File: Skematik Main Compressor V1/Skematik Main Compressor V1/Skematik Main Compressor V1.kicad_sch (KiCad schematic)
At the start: 4 parts, among them J1 Conn_01x04_Pin, U1 ESP32-WROOM-32UE

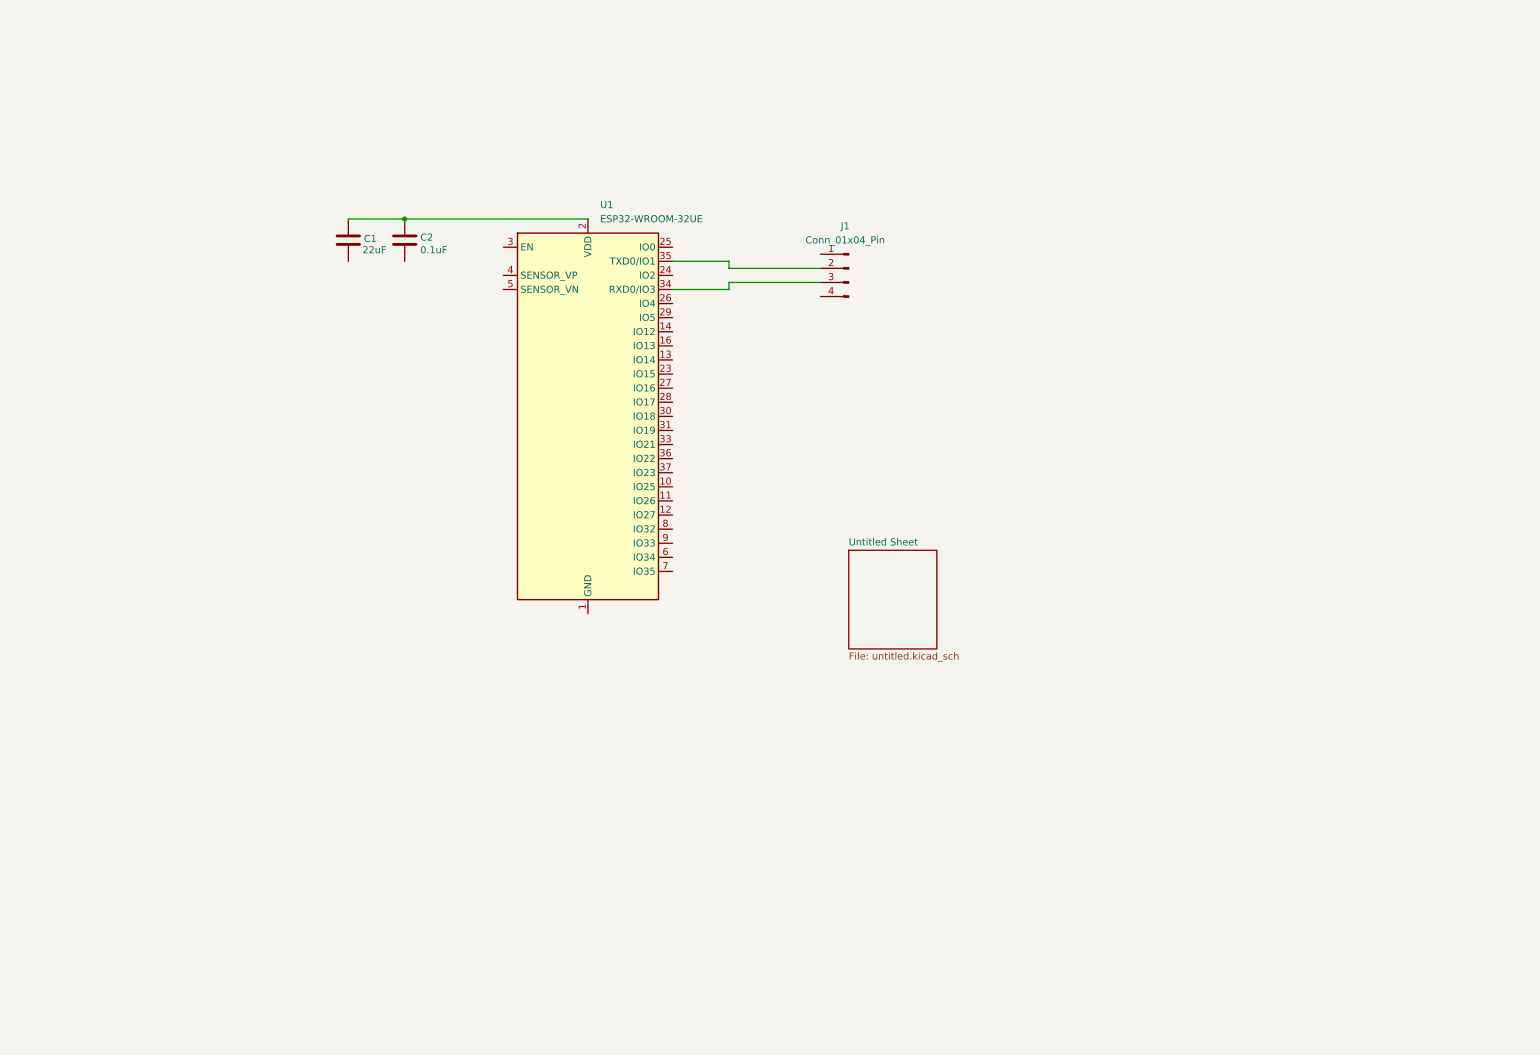
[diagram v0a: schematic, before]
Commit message: Update Main
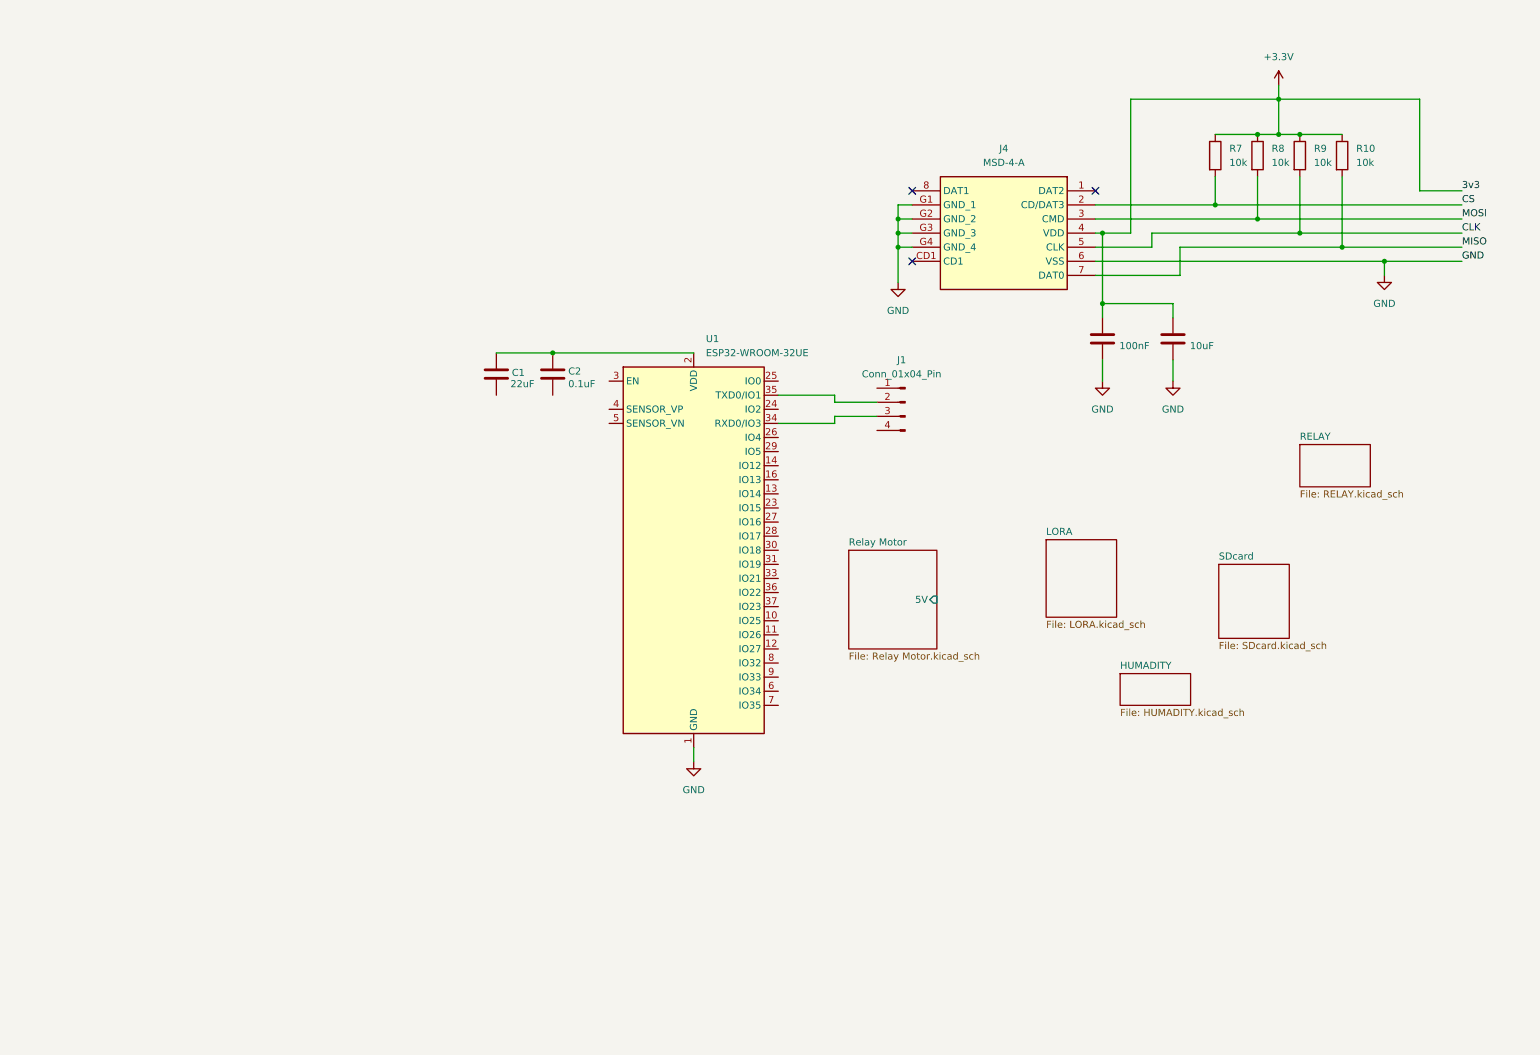
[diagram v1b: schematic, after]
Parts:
- added C5: 100nF, Capacitor_SMD:C_0504_1310Metric_Pad0.83x1.28mm_HandSolder, symbol Device:C
- added C6: 10uF, Capacitor_SMD:C_0504_1310Metric_Pad0.83x1.28mm_HandSolder, symbol Device:C
- added J4: MSD-4-A, MSD4A, symbol MSD-4-A:MSD-4-A
- added R10, R7, R8, R9: 10k, Resistor_SMD:R_0402_1005Metric_Pad0.72x0.64mm_HandSolder, symbol Device:R
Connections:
- net GND: now reaches U1.1 (GND), U1.15 (GND), U1.38 (GND), U1.39 (GND)
- net GND: now also C5.2, C6.2, J4.6 (VSS), J4.G1 (GND_1), J4.G2 (GND_2), J4.G3 (GND_3), J4.G4 (GND_4)
- new net +3.3V: C5.1, C6.1, J4.4 (VDD), R10.1, R7.1, R8.1, R9.1
- new net CLK: J4.5 (CLK), R9.2
- new net CS: J4.2 (CD/DAT3), R7.2
- new net MISO: J4.7 (DAT0), R10.2
- new net MOSI: J4.3 (CMD), R8.2
- no-connect marks 0 -> 3
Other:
- sheet Untitled Sheet renamed Relay Motor
- added sheet HUMADITY (HUMADITY.kicad_sch)
- added sheet LORA (LORA.kicad_sch)
- added sheet RELAY (RELAY.kicad_sch)
- added sheet SDcard (SDcard.kicad_sch)
- sheet Relay Motor: file untitled.kicad_sch -> Relay Motor.kicad_sch
- sheet Relay Motor ports: added 5V; removed none
- moved on the sheet: C1, C2, J1, U1

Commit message: Penambahan Skematik Main Compressor V1
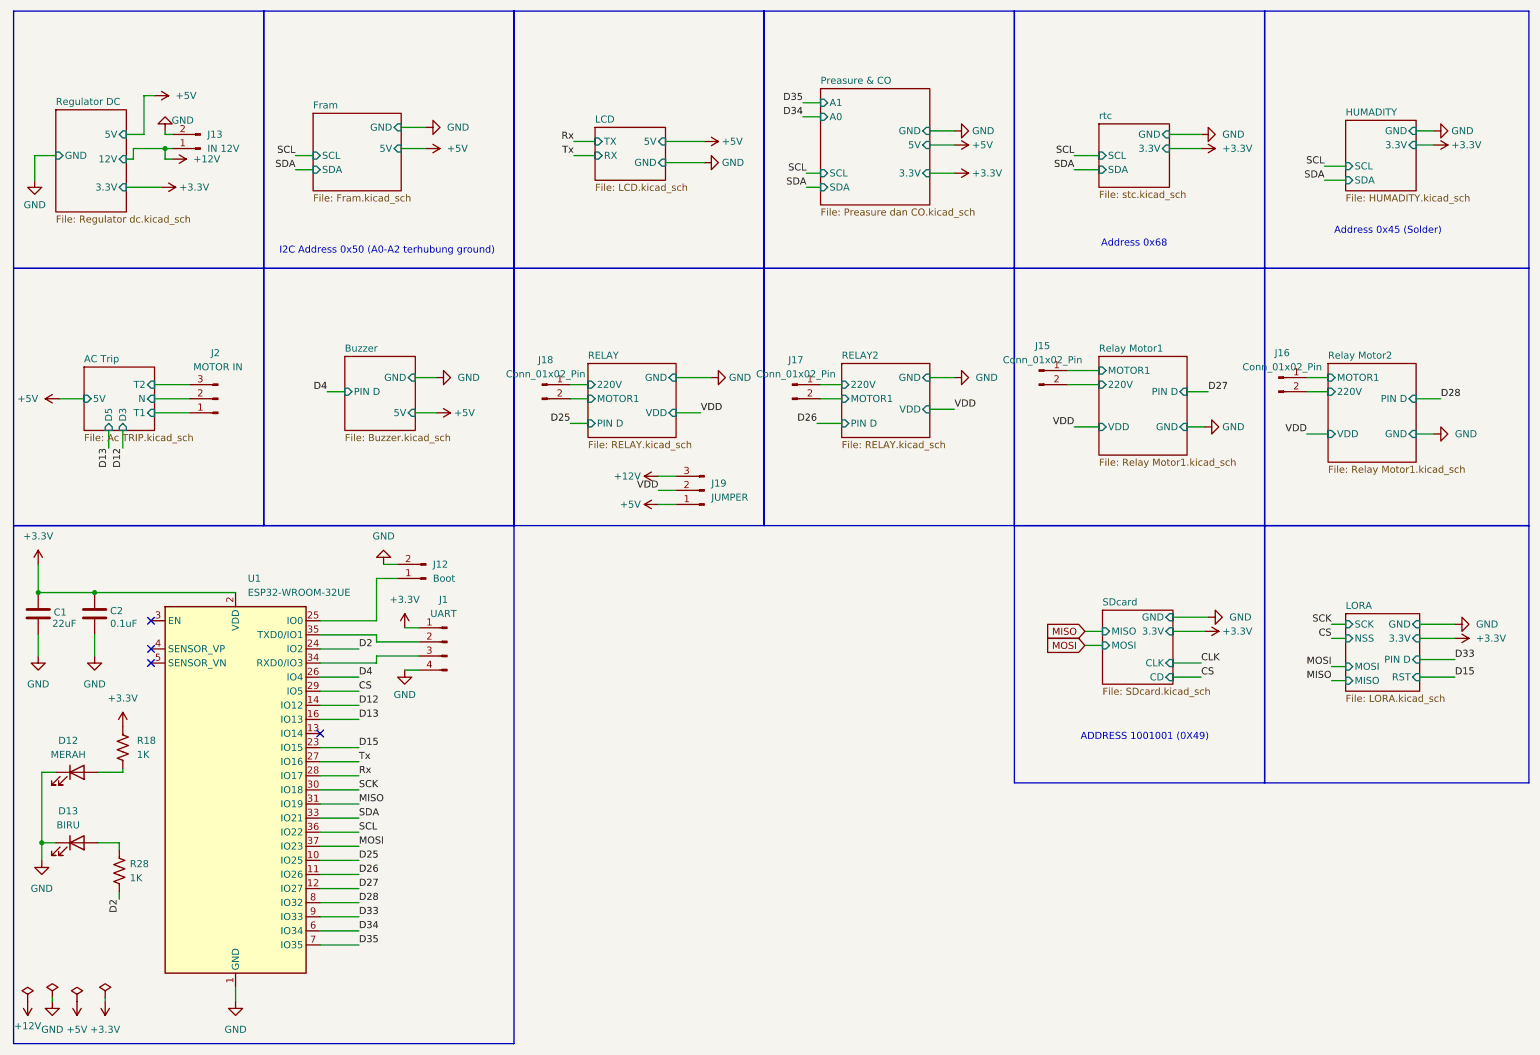
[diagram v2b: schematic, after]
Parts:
- removed C5: 100nF, Capacitor_SMD:C_0504_1310Metric_Pad0.83x1.28mm_HandSolder, symbol Device:C
- removed C6: 10uF, Capacitor_SMD:C_0504_1310Metric_Pad0.83x1.28mm_HandSolder, symbol Device:C
- removed J4: MSD-4-A, MSD4A, symbol MSD-4-A:MSD-4-A
- removed R10, R7, R8, R9: 10k, Resistor_SMD:R_0402_1005Metric_Pad0.72x0.64mm_HandSolder, symbol Device:R
- added D12: MERAH, LED_SMD:LED_0402_1005Metric_Pad0.77x0.64mm_HandSolder, symbol Device:LED
- added D13: BIRU, LED_SMD:LED_0402_1005Metric_Pad0.77x0.64mm_HandSolder, symbol Device:LED
- added J12: Boot, Connector_PinHeader_2.54mm:PinHeader_1x02_P2.54mm_Vertical, symbol Connector:Conn_01x02_Pin
- added J13: IN 12V, Connector_Molex:Molex_KK-396_A-41791-0002_1x02_P3.96mm_Vertical, symbol Connector:Conn_01x02_Pin
- added J15, J16, J17, J18: Conn_01x02_Pin, Connector_Molex:Molex_KK-396_A-41791-0002_1x02_P3.96mm_Vertical, symbol Connector:Conn_01x02_Pin
- added J19: JUMPER, Connector_PinHeader_2.54mm:PinHeader_1x03_P2.54mm_Vertical, symbol Connector:Conn_01x03_Pin
- added J2: MOTOR IN, Connector_Molex:Molex_KK-396_A-41791-0003_1x03_P3.96mm_Vertical, symbol Connector:Conn_01x03_Pin
- added R18, R28: 1K, Resistor_SMD:R_0402_1005Metric_Pad0.72x0.64mm_HandSolder, symbol Device:R_US
- J1: value Conn_01x04_Pin -> UART
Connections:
- net +3.3V: now also C1.1, C2.1, J1.1 (Pin_1), U1.2 (VDD), R18.1
- net CS: now also U1.29 (IO5)
- net GND: now also C1.2, C2.2, J1.4 (Pin_4), D12.1 (K), D13.1 (K), J12.2 (Pin_2), J13.2 (Pin_2)
- net MISO: now also U1.31 (IO19)
- net MOSI: now also U1.37 (IO23)
- net D25: now reaches U1.10 (IO25)
- net D26: now reaches U1.11 (IO26)
- net D27: now reaches U1.12 (IO27)
- net D12: now reaches U1.14 (IO12)
- net D13: now reaches U1.16 (IO13)
- net D15: now reaches U1.23 (IO15)
- net D2: now reaches U1.24 (IO2)
- net D2: now also R28.2
- net at U1.25 (IO0): now also J12.1 (Pin_1)
- net D4: now reaches U1.26 (IO4)
- net Tx: now reaches U1.27 (IO16)
- net Rx: now reaches U1.28 (IO17)
- net SCK: now reaches U1.30 (IO18)
- net SDA: now reaches U1.33 (IO21)
- net SCL: now reaches U1.36 (IO22)
- net D34: now reaches U1.6 (IO34)
- net D35: now reaches U1.7 (IO35)
- net D28: now reaches U1.8 (IO32)
- net D33: now reaches U1.9 (IO33)
- new net: D13.2 (A), R28.1
- new net: D12.2 (A), R18.2
- new net +12V: J13.1 (Pin_1), J19.3 (Pin_3)
- new net +5V: J19.1 (Pin_1)
- new net AC Trip/N: J2.2 (Pin_2)
- new net AC Trip/T1: J2.1 (Pin_1)
- new net AC Trip/T2: J2.3 (Pin_3)
- new net RELAY/220V: J18.1 (Pin_1)
- new net RELAY/MOTOR1: J18.2 (Pin_2)
- new net RELAY2/220V: J17.1 (Pin_1)
- new net RELAY2/MOTOR1: J17.2 (Pin_2)
- new net Relay Motor1/220V: J15.2 (Pin_2)
- new net Relay Motor1/MOTOR1: J15.1 (Pin_1)
- new net Relay Motor2/220V: J16.2 (Pin_2)
- new net Relay Motor2/MOTOR1: J16.1 (Pin_1)
- new net VDD: J19.2 (Pin_2)
- no-connect marks 3 -> 4
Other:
- sheet Relay Motor renamed Relay Motor1
- added sheet AC Trip (Ac TRIP.kicad_sch)
- added sheet Buzzer (Buzzer.kicad_sch)
- added sheet Fram (Fram.kicad_sch)
- added sheet LCD (LCD.kicad_sch)
- added sheet Preasure & CO (Preasure dan CO.kicad_sch)
- added sheet RELAY2 (RELAY.kicad_sch)
- added sheet Regulator DC (Regulator dc.kicad_sch)
- added sheet Relay Motor2 (Relay Motor1.kicad_sch)
- added sheet rtc (stc.kicad_sch)
- sheet HUMADITY ports: added 3.3V, GND, SCL, SDA; removed none
- sheet LORA ports: added 3.3V, GND, MISO, MOSI, NSS, PIN D, RST, SCK; removed none
- sheet RELAY ports: added 220V, GND, MOTOR1, PIN D, VDD; removed none
- sheet Relay Motor1: file Relay Motor.kicad_sch -> Relay Motor1.kicad_sch
- sheet Relay Motor1 ports: added 220V, GND, MOTOR1, PIN D, VDD; removed 5V
- sheet SDcard ports: added 3.3V, CD, CLK, GND, MISO, MOSI; removed none
- note added: "ADDRESS 1001001 (0X49)"
- note added: "Address 0x45 (Solder)"
- note added: "Address 0x68"
- note added: "I2C Address 0x50 (A0-A2 terhubung ground)"
- moved on the sheet: C1, C2, J1, U1
